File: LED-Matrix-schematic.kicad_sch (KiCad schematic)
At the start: 67 parts, among them J1 Conn_02x07_Odd_Even_MountingP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, M200 74HC595, M201 74HC595

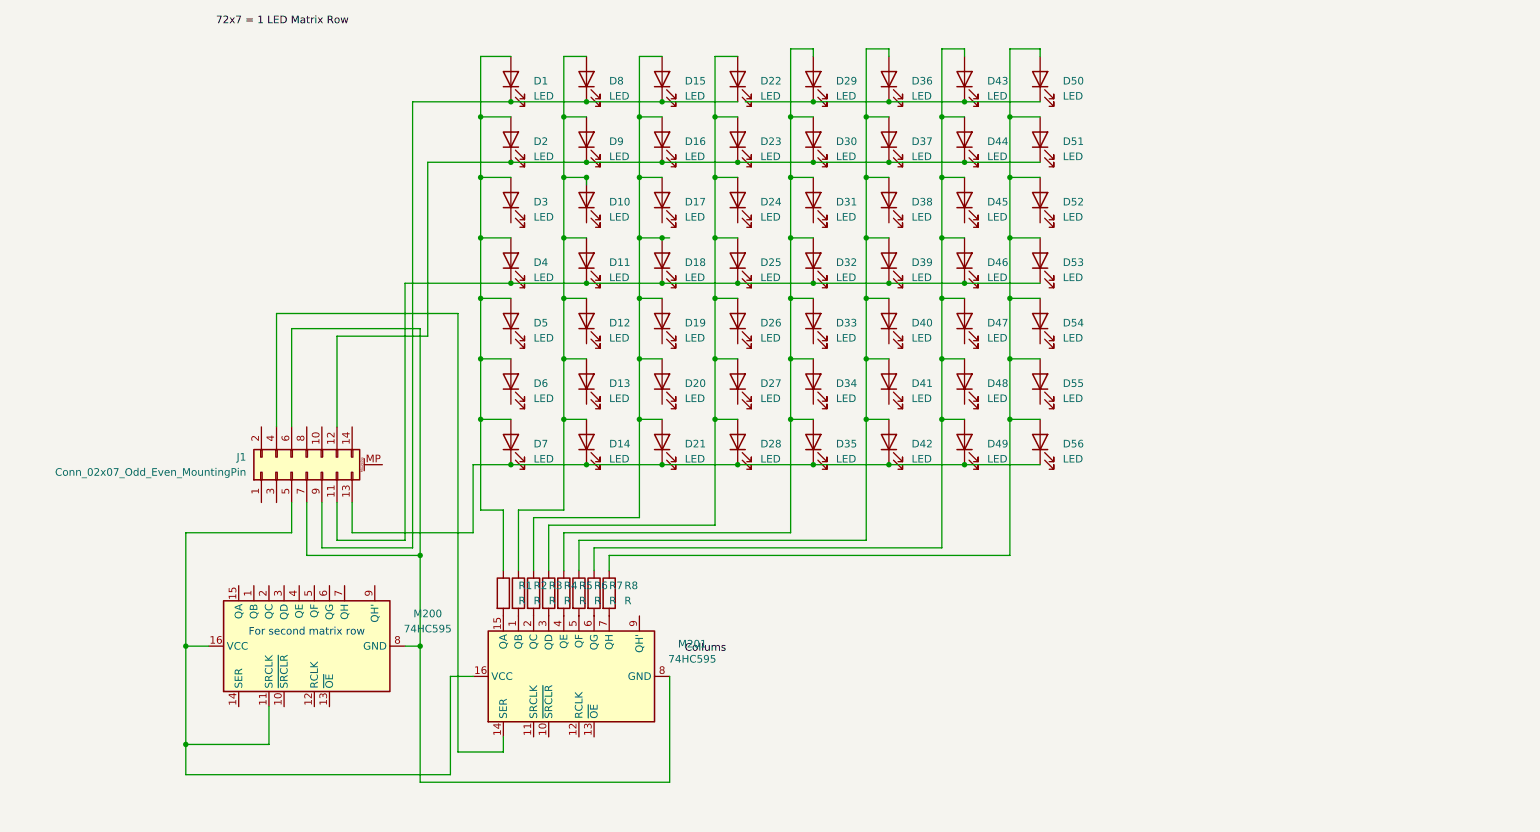
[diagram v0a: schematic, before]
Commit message: Updated schematic
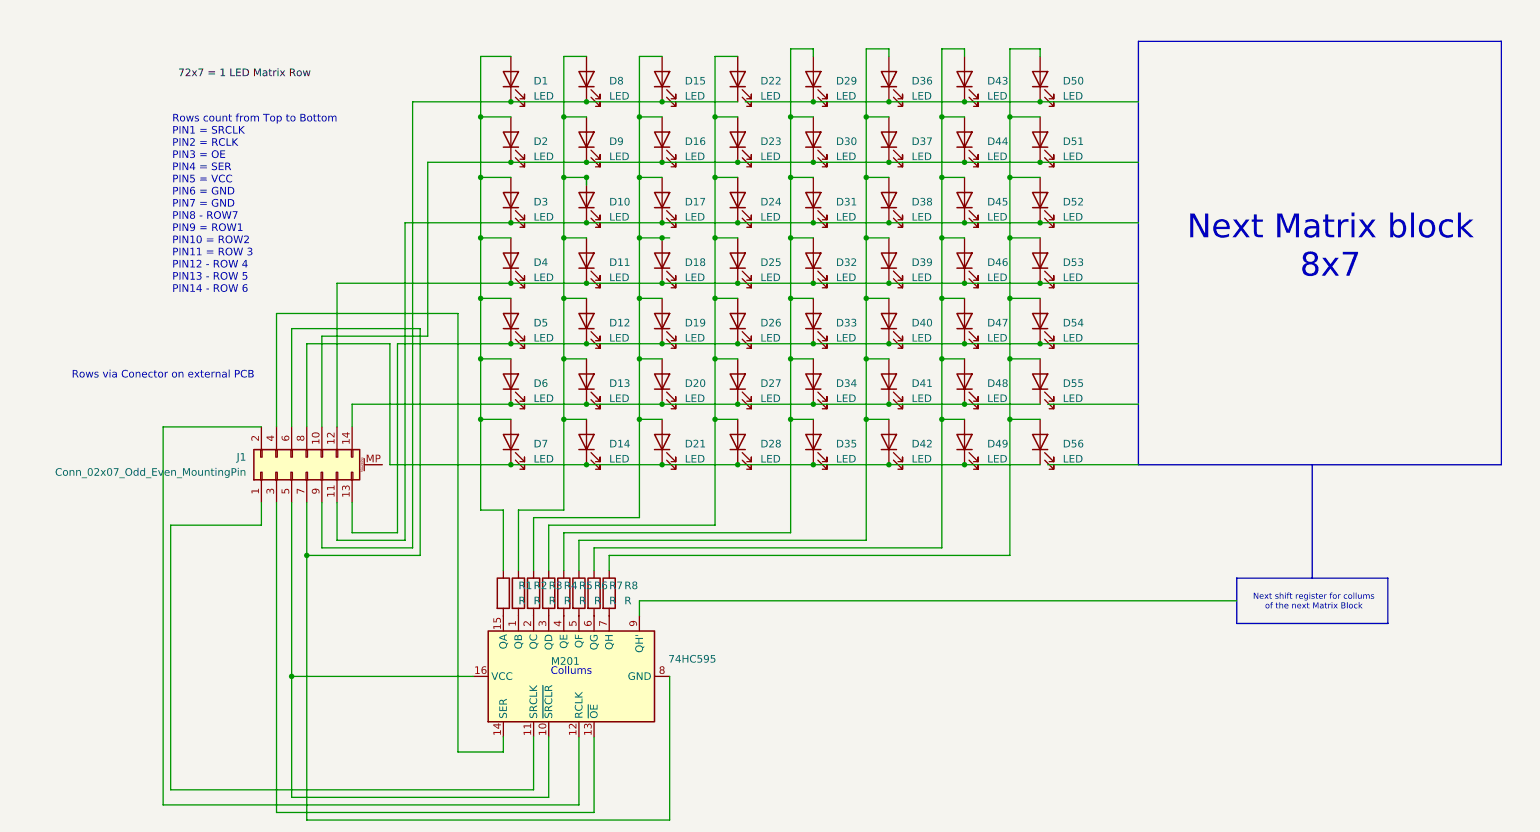
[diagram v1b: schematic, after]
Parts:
- removed M200: 74HC595, symbol 74xx:74HC595
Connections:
- net at D11.1 (K), D18.1 (K), D25.1 (K)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: now also J1.12 (Pin_12); no longer J1.11 (Pin_11)
- net at D40.1 (K): now also D12.1 (K), D19.1 (K), D26.1 (K), D33.1 (K), D47.1 (K), D5.1 (K), D54.1 (K), J1.13 (Pin_13)
- net at D16.1 (K), D2.1 (K), D23.1 (K)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: now also J1.10 (Pin_10); no longer J1.12 (Pin_12)
- net at D14.1 (K), D21.1 (K), D28.1 (K)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: now also J1.8 (Pin_8); no longer J1.13 (Pin_13)
- net at D20.1 (K): now also D13.1 (K), D27.1 (K), D34.1 (K), D41.1 (K), D48.1 (K), D55.1 (K), D6.1 (K), J1.14 (Pin_14)
- net at M201.10 (~{SRCLR}): now also J1.5 (Pin_5), M201.16 (VCC)
- net at M201.11 (SRCLK): now also J1.1 (Pin_1)
- net at M201.12 (RCLK): now also J1.2 (Pin_2)
- net at M201.13 (~{OE}): now also J1.3 (Pin_3)
- net at D31.1 (K): now also D10.1 (K), D17.1 (K), D24.1 (K), D3.1 (K), D38.1 (K), D45.1 (K), D52.1 (K), J1.11 (Pin_11)
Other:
- note added: "Collums"
- note added: "Next Matrix block 8x7"
- note added: "Next shift register for collums of the next Matrix Block"
- note added: "Rows count from Top to Bottom PIN1 = SRCLK PIN2 = RCLK PIN3 = OE PIN4 = SER PIN5 = VCC PIN6 = GND PIN7 = GND PIN8 - ROW7 PIN9 = ROW1 PIN10 = ROW2 PIN11 = ROW 3 PIN12 - ROW 4 PIN13 - ROW 5 PIN14 - ROW 6"
- note added: "Rows via Conector on external PCB"
- note removed: "For second matrix row"
